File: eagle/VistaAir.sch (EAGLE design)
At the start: 6 parts

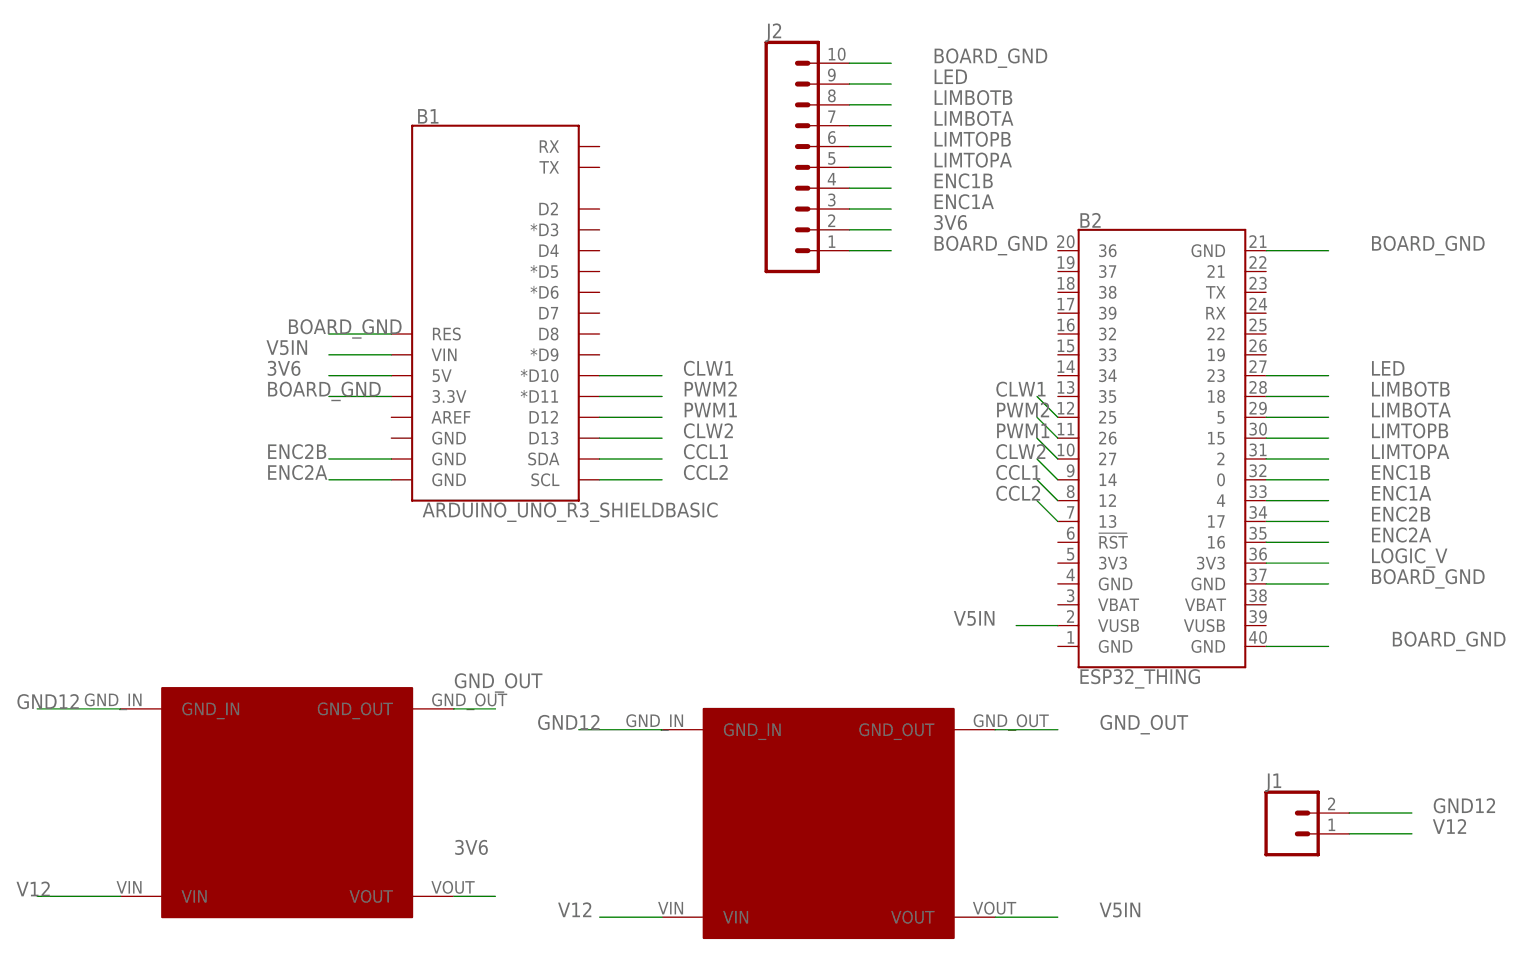
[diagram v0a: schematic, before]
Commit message: pcb corrections
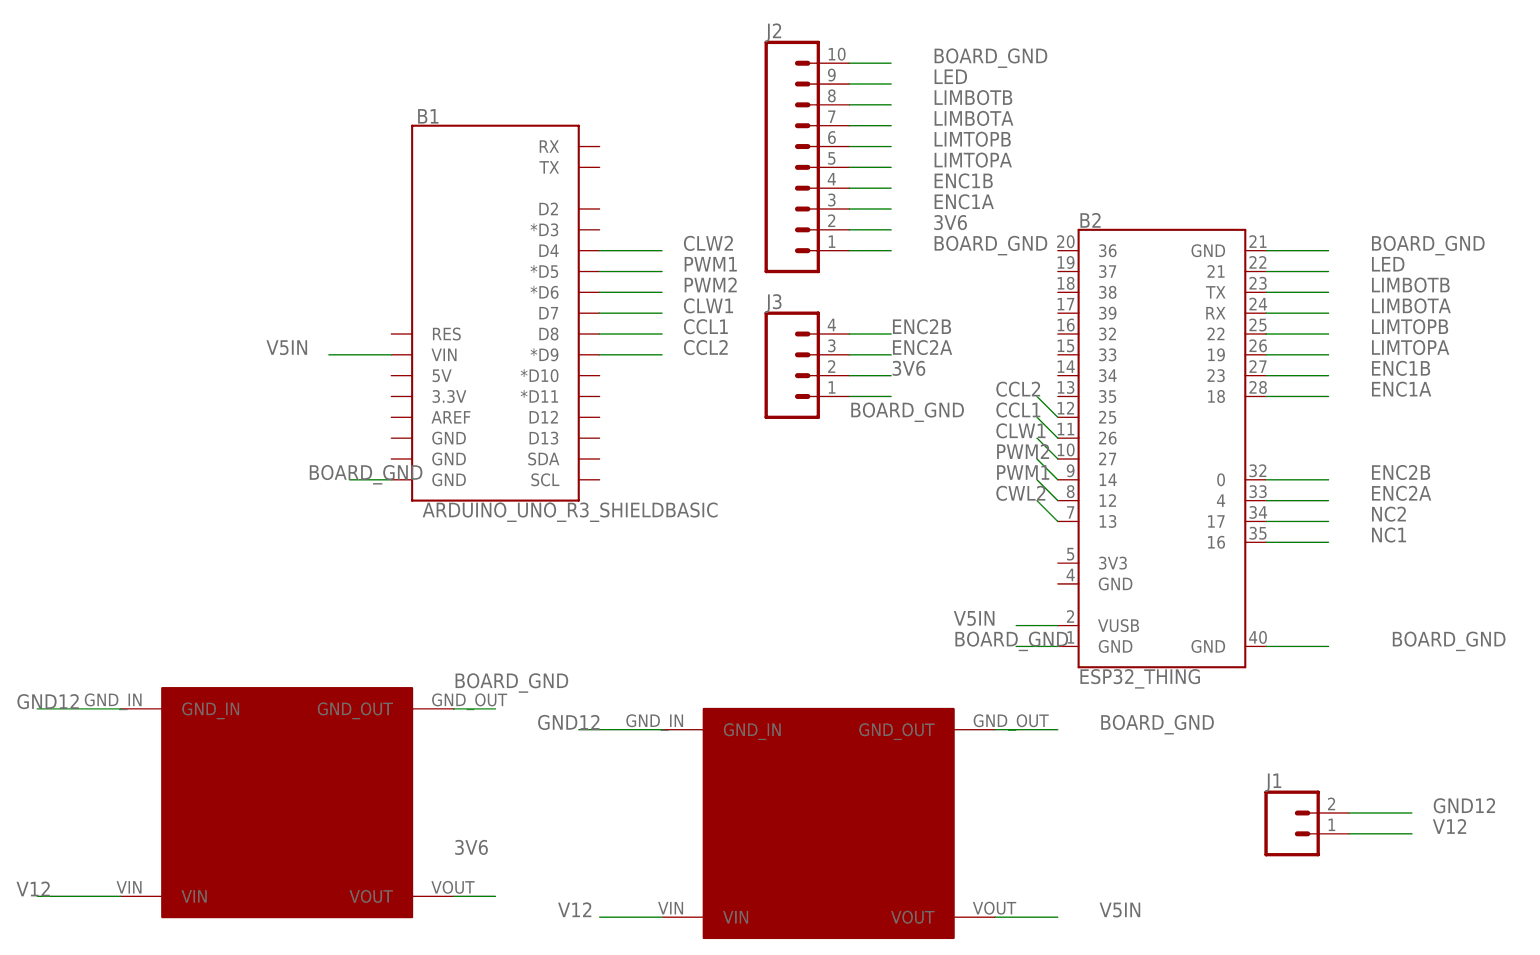
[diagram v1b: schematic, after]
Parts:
- added J3: (no value), SparkFun-Connectors:CONN_04
- B2: device SparkFun-Boards:ESP32_THING -> kevins_parts:ESP32_THING
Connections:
- removed net GND_OUT: U$1.GND_OUT, U$2.GND_OUT
- removed net LOGIC_V: B2.3V3@36
- new net CWL2: B2.13
- new net NC1: B2.16
- new net NC2: B2.17
- net 3V6: now also J3.2; no longer B1.5V
- net BOARD_GND: now also B1.GND@0, B2.GND@1, J3.1, U$1.GND_OUT, U$2.GND_OUT; no longer B1.3.3V, B1.RES, B2.GND@37
- net CCL1: now also B1.D8, B2.26; no longer B1.SDA, B2.12
- net CCL2: now also B1.*D9, B2.25; no longer B1.SCL, B2.13
- net CLW1: now also B1.D7, B2.27; no longer B1.*D10, B2.25
- net CLW2: now also B1.D4; no longer B1.D13, B2.14
- net ENC1A: now also B2.18; no longer B2.4
- net ENC1B: now also B2.23; no longer B2.0
- net ENC2A: now also B2.4, J3.3; no longer B1.GND@0, B2.16
- net ENC2B: now also B2.0, J3.4; no longer B1.GND@1, B2.17
- net LED: now also B2.21; no longer B2.23
- net LIMBOTA: now also B2.RX; no longer B2.5
- net LIMBOTB: now also B2.TX; no longer B2.18
- net LIMTOPA: now also B2.19; no longer B2.2
- net LIMTOPB: now also B2.22; no longer B2.15
- net PWM1: now also B1.*D5, B2.12; no longer B1.D12, B2.27
- net PWM2: now also B1.*D6, B2.14; no longer B1.*D11, B2.26
